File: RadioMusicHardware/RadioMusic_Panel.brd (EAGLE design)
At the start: 128.5 x 20 mm, 0 parts

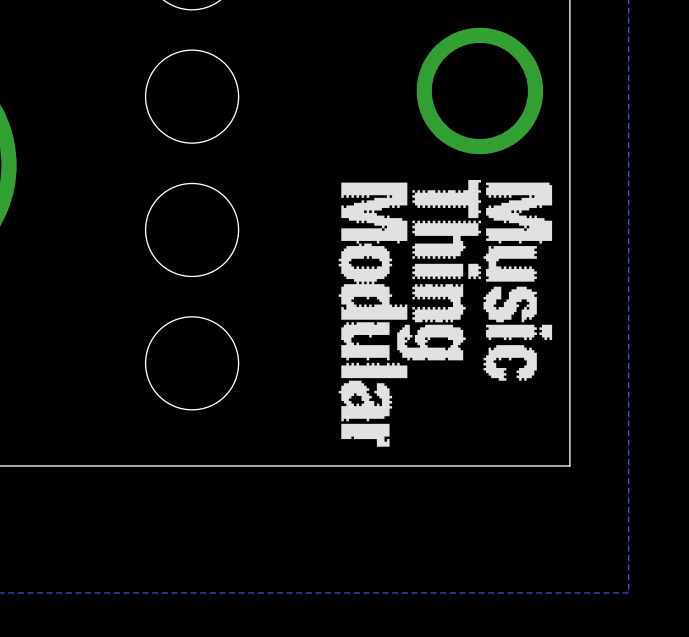
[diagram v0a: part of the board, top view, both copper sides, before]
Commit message: Text subbing
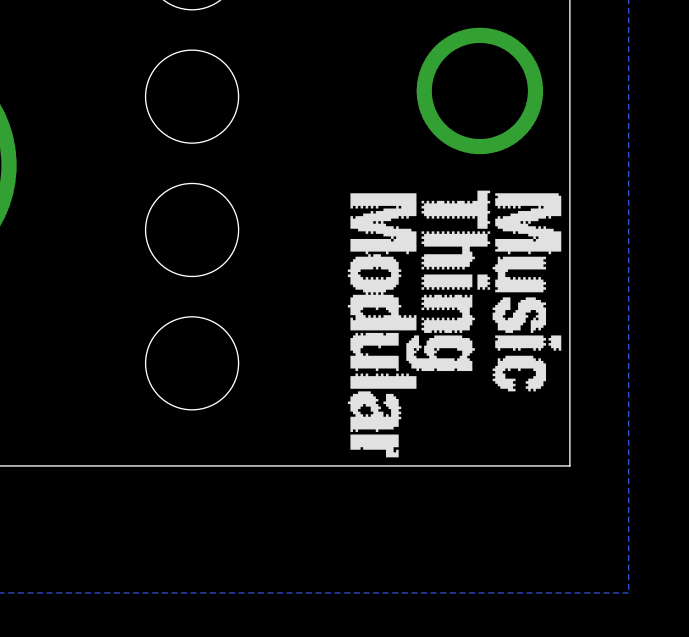
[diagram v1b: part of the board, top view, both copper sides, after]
